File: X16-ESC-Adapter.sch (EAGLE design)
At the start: 4 parts, among them J1 CONN_1824750000

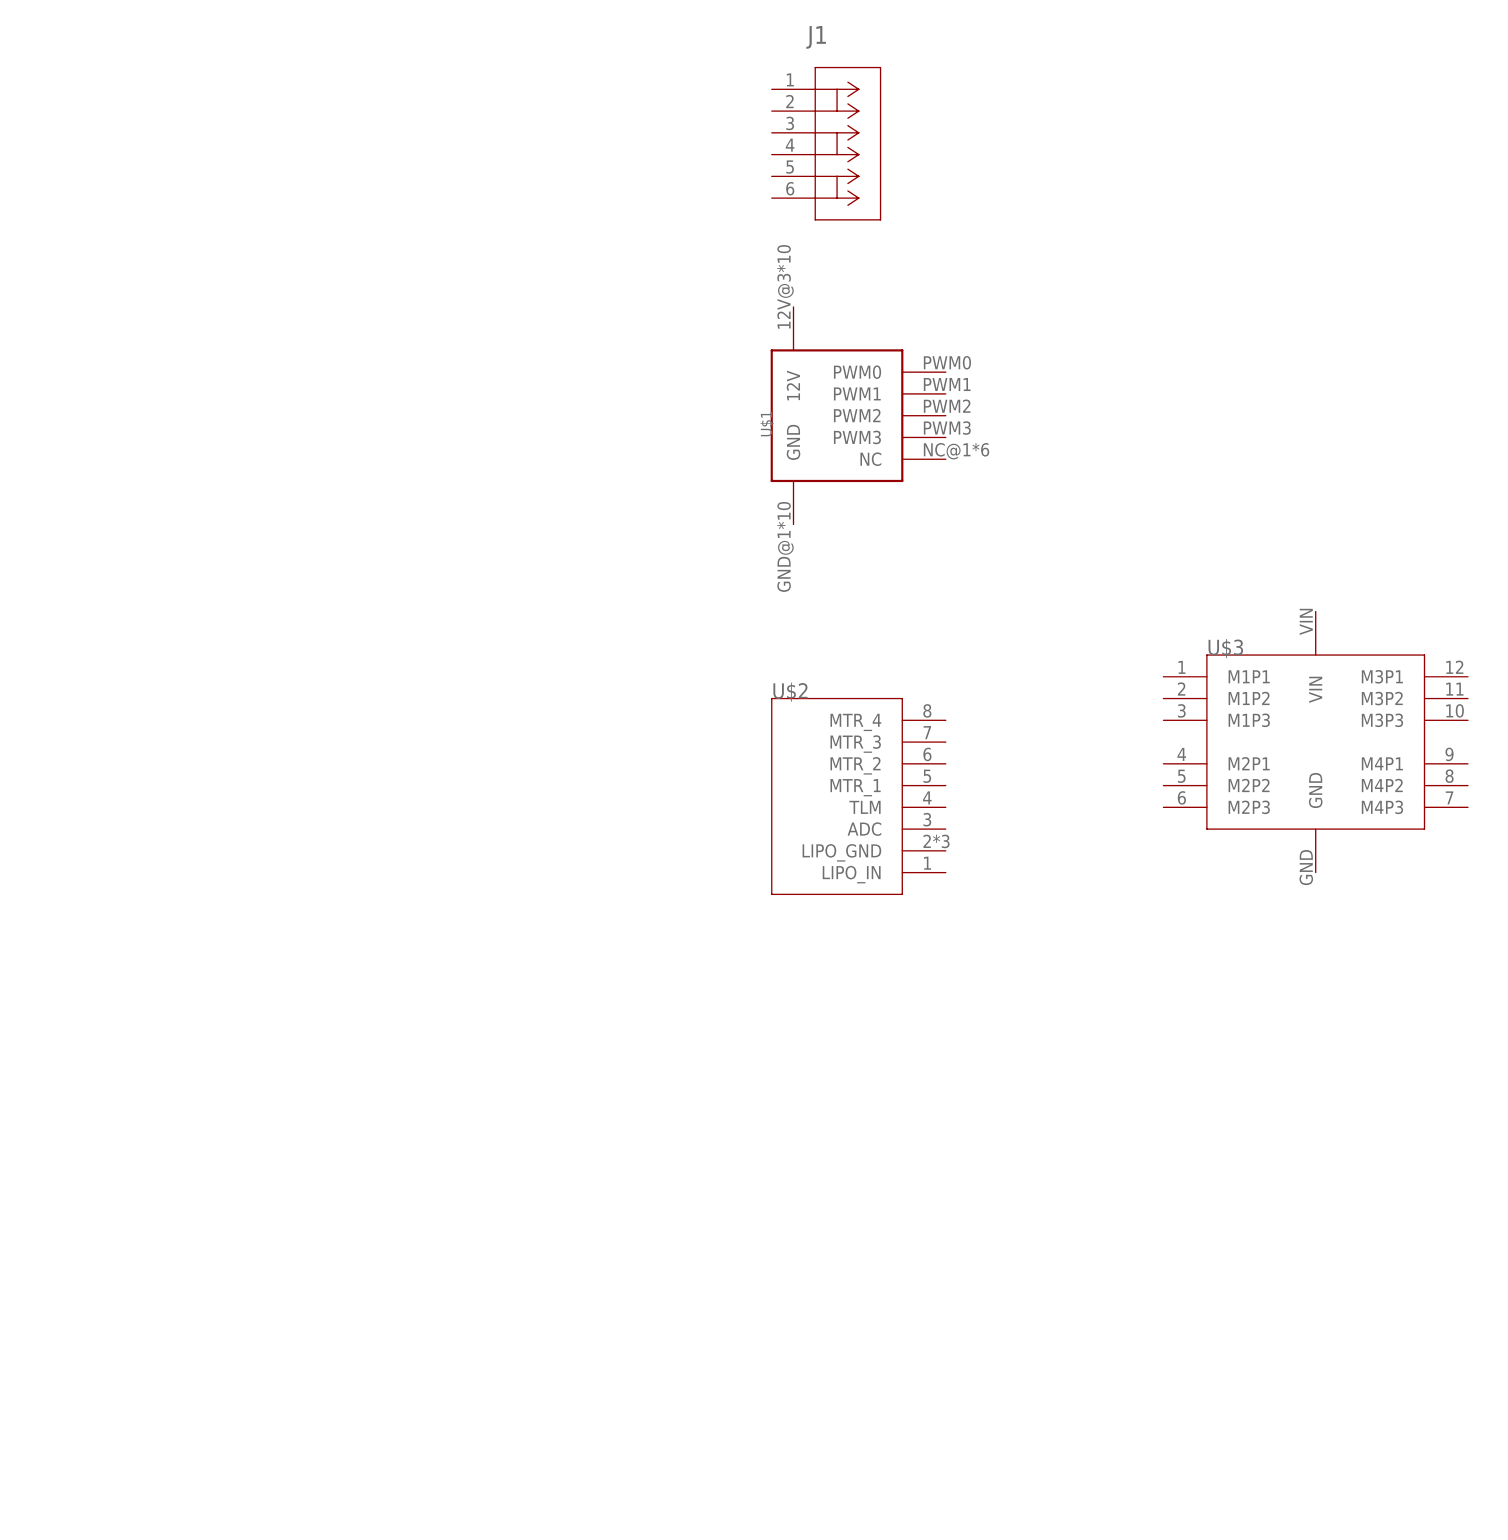
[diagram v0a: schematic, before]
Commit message: Curren tprogress on schem
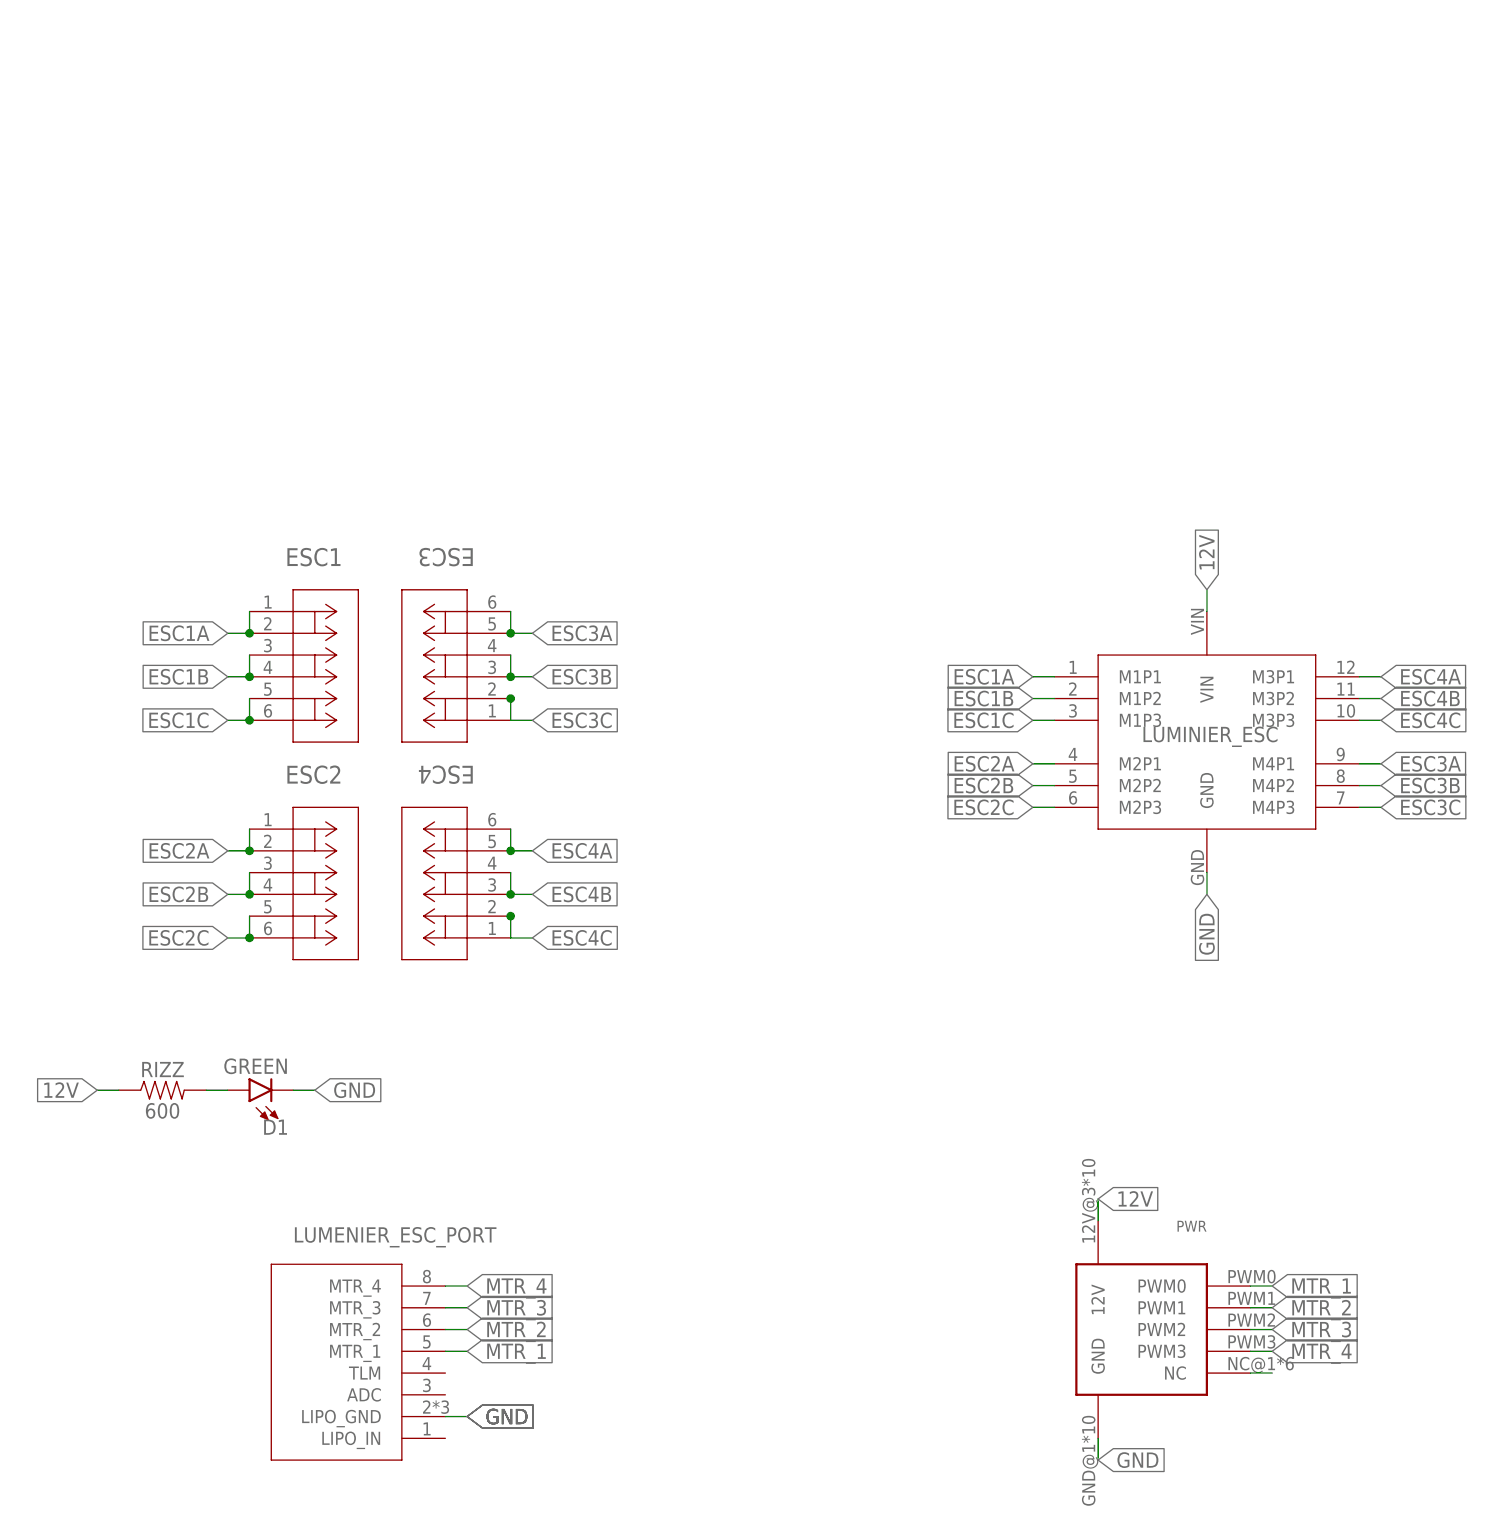
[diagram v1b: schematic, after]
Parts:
- removed J1: CONN_1824750000, X16-ESC-Adapter:CONN_1824750000
- removed U$1: CONN_BACKPLANE_ESC_ADAPTER, X16-ESC-Adapter:CONN_BACKPLANE_ESC_ADAPTER
- removed U$2: CONN_JST_8_PIN, X16-ESC-Adapter:CONN_JST_8_PIN
- removed U$3: LUMENIER, X16-ESC-Adapter:LUMENIER
- added D1: GREEN, SparkFun-LED:LED0603
- added ESC1, ESC2, ESC3, ESC4: CONN_1824750000, X16-ESC-Adapter:CONN_1824750000
- added LUMENIER_ESC_PORT: CONN_JST_8_PIN, X16-ESC-Adapter:CONN_JST_8_PIN
- added LUMINIER_ESC: LUMENIER, X16-ESC-Adapter:LUMENIER
- added PWR: CONN_BACKPLANE_ESC_ADAPTER, X16-ESC-Adapter:CONN_BACKPLANE_ESC_ADAPTER
- added RIZZ: 600, SparkFun-Resistors:0.1OHM-0603-1/3W-1%
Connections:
- new net 12V: LUMINIER_ESC.VIN, PWR.12V, RIZZ.1
- new net ESC1A: ESC1.1, ESC1.2, LUMINIER_ESC.M1P1
- new net ESC1B: ESC1.3, ESC1.4, LUMINIER_ESC.M1P2
- new net ESC1C: ESC1.5, ESC1.6, LUMINIER_ESC.M1P3
- new net ESC2A: ESC2.1, ESC2.2, LUMINIER_ESC.M2P1
- new net ESC2B: ESC2.3, ESC2.4, LUMINIER_ESC.M2P2
- new net ESC2C: ESC2.5, ESC2.6, LUMINIER_ESC.M2P3
- new net ESC3A: ESC3.5, ESC3.6, LUMINIER_ESC.M4P1
- new net ESC3B: ESC3.3, ESC3.4, LUMINIER_ESC.M4P2
- new net ESC3C: ESC3.1, ESC3.2, LUMINIER_ESC.M4P3
- new net ESC4A: ESC4.5, ESC4.6, LUMINIER_ESC.M3P1
- new net ESC4B: ESC4.3, ESC4.4, LUMINIER_ESC.M3P2
- new net ESC4C: ESC4.1, ESC4.2, LUMINIER_ESC.M3P3
- new net GND: D1.C, LUMENIER_ESC_PORT.LIPO_GND, LUMINIER_ESC.GND, PWR.GND
- new net MTR_1: LUMENIER_ESC_PORT.MTR_1, PWR.PWM0
- new net MTR_2: LUMENIER_ESC_PORT.MTR_2, PWR.PWM1
- new net MTR_3: LUMENIER_ESC_PORT.MTR_3, PWR.PWM2
- new net MTR_4: LUMENIER_ESC_PORT.MTR_4, PWR.PWM3
- new net N$1: D1.A, RIZZ.2
- new net N$7: PWR.NC
